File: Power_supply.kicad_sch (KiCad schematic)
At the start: 16 parts, among them J2 DC_DC_Buck_converter_module, U1 TPS562201DDCR

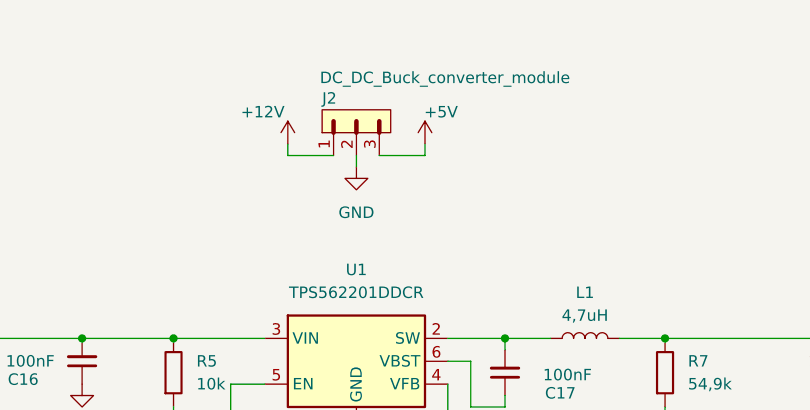
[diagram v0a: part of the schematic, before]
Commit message: wip
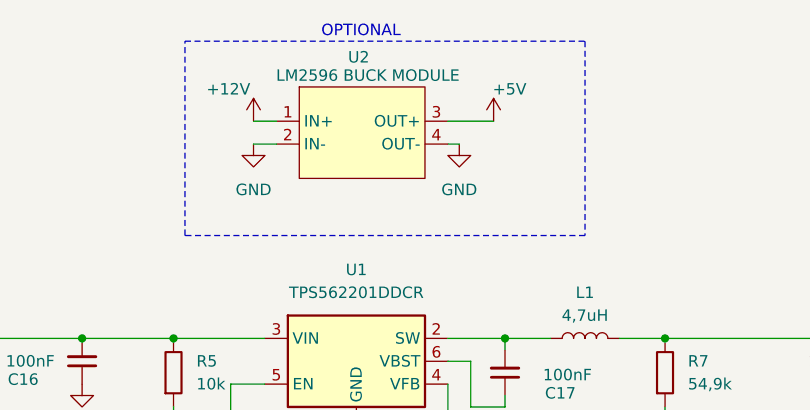
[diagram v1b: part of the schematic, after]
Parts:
- removed J2: DC_DC_Buck_converter_module, Connector_PinHeader_2.54mm:PinHeader_1x03_P2.54mm_Vertical, symbol PCM_SL_Pin_Headers:PINHD_1x3_Male
- added U2: LM2596 BUCK MODULE, footprint_lib:LM2596 DC-DC module, symbol sym_lib:DC-DC_Step_down_module
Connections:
- net +12V: now also U2.1 (IN+)
- net +5V: now also U2.3 (OUT+)
- net GND: now also U2.2 (IN-), U2.4 (OUT-)
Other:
- note added: "OPTIONAL"
